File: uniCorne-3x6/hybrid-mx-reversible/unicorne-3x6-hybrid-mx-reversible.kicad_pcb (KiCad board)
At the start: 2 copper layers, 133.8 x 91.4 mm, 100 parts, among them J1 MJ-4PP-9, J2 Nice!View, J3 Conn_01x02, J4 Conn_01x03, SW1 SW_MX_HS, SW10 SW_MX_HS, SW11 SW_MX_HS, SW12 SW_MX_HS, SW13 SW_MX_HS, SW14 SW_MX_HS, SW15 SW_MX_HS, SW16 SW_MX_HS, SW17 SW_MX_HS, SW18 SW_MX_HS, SW19 SW_CHOC_HS, SW2 SW_MX_HS, SW20 SW_CHOC_HS, SW21 SW_CHOC_HS, SW3 SW_MX_HS, SW4 SW_MX_HS, SW5 SW_MX_HS, SW6 SW_MX_HS, SW7 SW_MX_HS, SW8 SW_MX_HS, SW9 SW_MX_HS, U1 ProMicro-ish

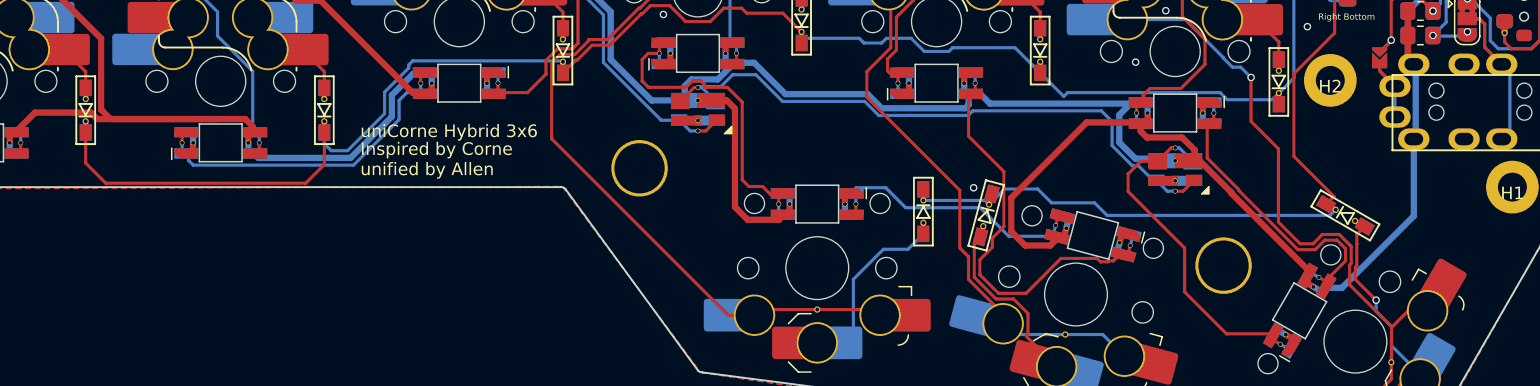
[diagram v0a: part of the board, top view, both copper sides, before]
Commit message: added more docs
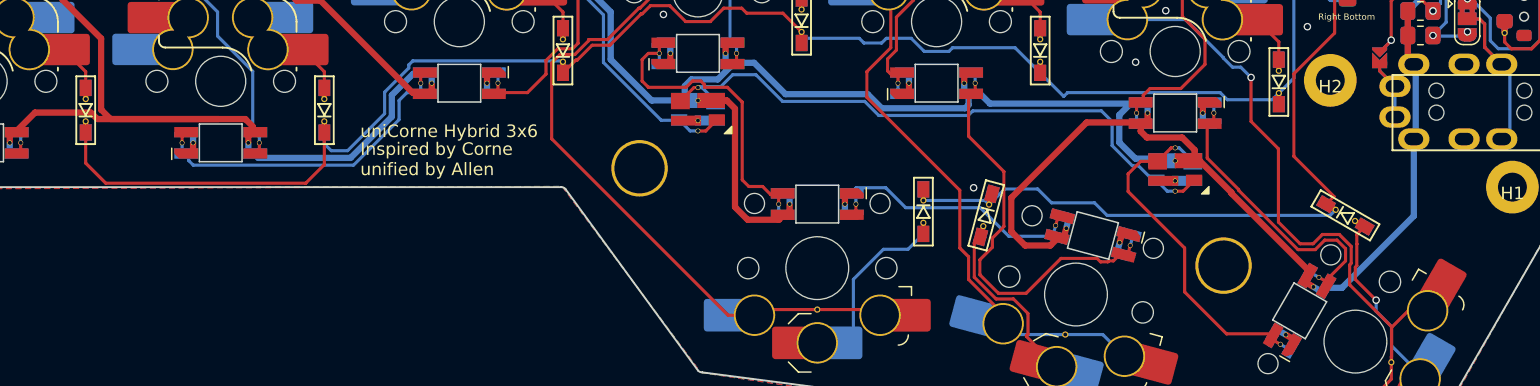
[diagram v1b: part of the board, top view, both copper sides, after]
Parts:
- D13, D14: moved to F.Cu
